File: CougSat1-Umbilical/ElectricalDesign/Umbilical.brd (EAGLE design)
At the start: 49 x 48 mm, 54 parts, among them J1 USB, J2 Umbilical, J3 5V input, Q1 CSD16406Q3, Q2 CSD16406Q3, U1 FT230XQ, U2 BQ24650

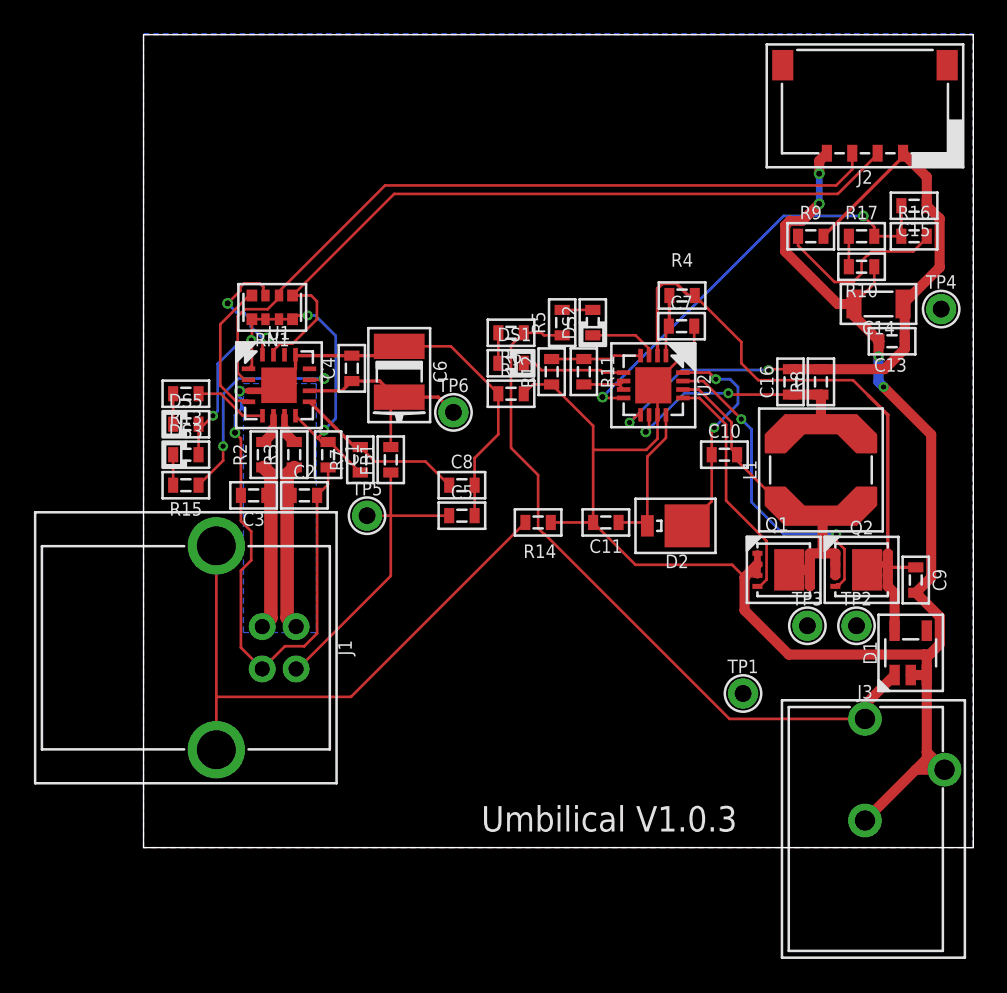
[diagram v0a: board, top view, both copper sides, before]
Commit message: Updated Umbilical
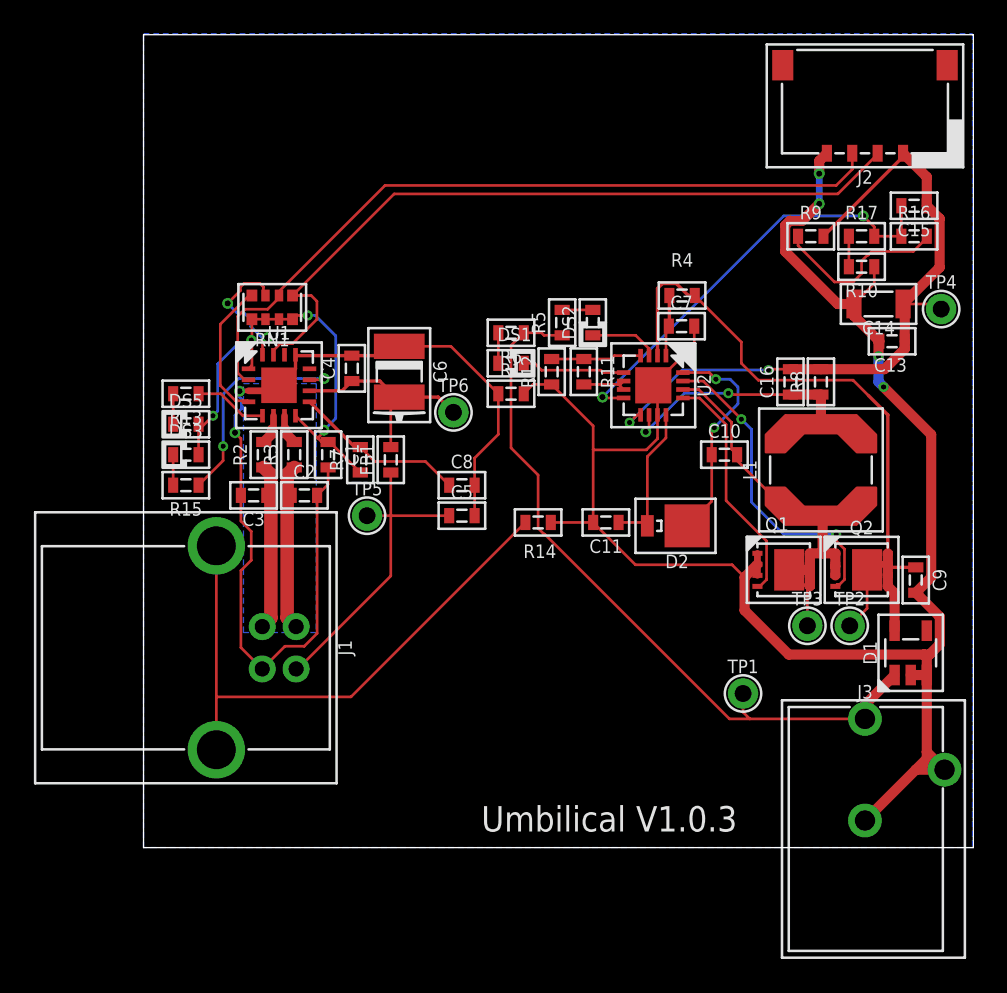
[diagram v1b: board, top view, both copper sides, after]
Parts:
- moved TP2 0.40 mm to (41.7, 13.1)
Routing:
- net PH: track 21.6 -> 25.6 mm
- net DIODE_OUT: track 39.2 -> 42.9 mm
- net UMB_OUT: track 39.2 -> 41.6 mm
- net 5.0V: track 42.4 -> 43.8 mm
- removed copper zone on layer 1, net BALANCING-TOP
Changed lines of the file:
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@@
 <attribute name="NAME" x="35.4" y="10.7" size="0.8" layer="25" font="vector" ratio="15" align="center"/>
 </element>
-<element name="TP2" library="CougsInSpace-Connectors" package="THT-1.0" value="TEST_POINT-THT-1.0" x="42.1" y="13.1" smashed="yes">
-<attribute name="NAME" x="42.1" y="14.7" size="0.8" layer="25" font="vector" ratio="15" align="center"/>
+<element name="TP2" library="CougsInSpace-Connectors" package="THT-1.0" value="TEST_POINT-THT-1.0" x="41.7" y="13.1" smashed="yes">
+<attribute name="NAME" x="41.7" y="14.7" size="0.8" layer="25" font="vector" ratio="15" align="center"/>
 </element>
 <element name="TP3" library="CougsInSpace-Connectors" package="THT-1.0" value="TEST_POINT-THT-1.0" x="39.2" y="13.1" smashed="yes">
@@
 <wire x1="35.3" y1="28.6" x2="36.3" y2="27.6" width="0.16" layer="1"/>
 <wire x1="36.3" y1="27.6" x2="41.9" y2="27.6" width="0.16" layer="1"/>
-<wire x1="42.1" y1="13.1" x2="44.35" y2="12.81" width="0" layer="19" extent="1-1"/>
+<wire x1="42.725" y1="16.4" x2="42.725" y2="14.125" width="0.16" layer="1"/>
+<wire x1="42.725" y1="14.125" x2="41.7" y2="13.1" width="0.16" layer="1"/>
 </signal>
 <signal name="BTST">
@@
 <contactref element="J3" pad="1"/>
 <contactref element="TP1" pad="1"/>
-<wire x1="44.35" y1="10.19" x2="44.26" y2="10.1" width="0.4" layer="1"/>
-<wire x1="22.57" y1="30.4" x2="22.45" y2="30.4" width="0.16" layer="1"/>
 <wire x1="42.6" y1="7.6" x2="42.6" y2="8.44" width="0.6" layer="1"/>
 <wire x1="42.6" y1="8.44" x2="44.35" y2="10.19" width="0.6" layer="1"/>
@@
 <wire x1="23.5" y1="30.4" x2="23.65" y2="30.25" width="0.16" layer="1"/>
 <wire x1="22.45" y1="30.4" x2="23.5" y2="30.4" width="0.16" layer="1"/>
-<wire x1="42.6" y1="7.6" x2="34.6" y2="7.6" width="0.16" layer="1"/>
+<wire x1="42.6" y1="7.6" x2="35.8" y2="7.6" width="0.16" layer="1"/>
+<wire x1="35.8" y1="7.6" x2="34.6" y2="7.6" width="0.16" layer="1"/>
 <wire x1="23.69" y1="18.51" x2="23.6505875" y2="18.51" width="0.16" layer="1"/>
 <wire x1="23.6505875" y1="18.51" x2="23.3" y2="18.8605875" width="0.16" layer="1"/>
@@
 <wire x1="23.3" y1="22" x2="21.7" y2="23.6" width="0.16" layer="1"/>
 <wire x1="21.7" y1="23.6" x2="21.7" y2="29.65" width="0.16" layer="1"/>
-<wire x1="42.6" y1="7.6" x2="35.4" y2="9.1" width="0" layer="19" extent="1-1"/>
+<wire x1="35.8" y1="7.6" x2="35.4" y2="8" width="0.16" layer="1"/>
+<wire x1="35.4" y1="8" x2="35.4" y2="9.1" width="0.16" layer="1"/>
 </signal>
 <signal name="CHARGING_STAT_G">
@@
 <contactref element="TP3" pad="1"/>
 <wire x1="40" y1="19.6" x2="39.0401875" y2="19.6" width="0.4" layer="1"/>
-<wire x1="40.85" y1="17.375" x2="40.85" y2="16.075" width="0.6" layer="1"/>
-<wire x1="39.35" y1="17.375" x2="39.35" y2="16.4" width="0.6" layer="1"/>
-<wire x1="39.35" y1="16.4" x2="39.35" y2="15.425" width="0.6" layer="1"/>
+<wire x1="40.85" y1="17.375" x2="40.85" y2="16.6" width="0.6" layer="1"/>
+<wire x1="40.85" y1="16.6" x2="40.85" y2="16.075" width="0.6" layer="1"/>
+<wire x1="39.35" y1="17.375" x2="39.35" y2="16.8" width="0.6" layer="1"/>
+<wire x1="39.35" y1="16.8" x2="39.35" y2="16.4" width="0.6" layer="1"/>
+<wire x1="39.35" y1="15.425" x2="39.35" y2="16" width="0.6" layer="1"/>
+<wire x1="39.35" y1="16" x2="39.35" y2="16.4" width="0.6" layer="1"/>
 <wire x1="38.125" y1="16.4" x2="39.35" y2="16.4" width="0.6" layer="1"/>
 <wire x1="40.85" y1="17.375" x2="40.1" y2="17.375" width="0.6" layer="1"/>
@@
 <wire x1="34.72" y1="23.53" x2="34.72" y2="25.11631875" width="0.16" layer="1"/>
 <wire x1="34.72" y1="25.11631875" x2="32.78631875" y2="27.05" width="0.16" layer="1"/>
-<wire x1="40.85" y1="16.075" x2="40.85" y2="16.725" width="0" layer="19" extent="1-1"/>
-<wire x1="39.35" y1="16.075" x2="39.35" y2="15.425" width="0" layer="19" extent="1-1"/>
-<wire x1="39.35" y1="16.725" x2="39.35" y2="17.375" width="0" layer="19" extent="1-1"/>
-<wire x1="39.2" y1="13.1" x2="39.35" y2="15.425" width="0" layer="19" extent="1-1"/>
+<wire x1="38.125" y1="16.4" x2="39.2" y2="15.325" width="0.16" layer="1"/>
+<wire x1="39.2" y1="15.325" x2="39.2" y2="13.1" width="0.16" layer="1"/>
+<wire x1="40.85" y1="16.725" x2="40.85" y2="16.6" width="0.16" layer="1"/>
+<wire x1="39.35" y1="16.725" x2="39.35" y2="16.8" width="0.16" layer="1"/>
+<wire x1="39.35" y1="16.075" x2="39.35" y2="16" width="0.16" layer="1"/>
 </signal>
 <signal name="HIGHDV">
@@
 <wire x1="36.9" y1="28.2" x2="36.95" y2="28.25" width="0.16" layer="1"/>
 <wire x1="36.95" y1="28.25" x2="38.2" y2="28.25" width="0.16" layer="1"/>
-<wire x1="44.85" y1="32.1" x2="47.1" y2="31.8" width="0" layer="19" extent="1-1"/>
+<wire x1="44.85" y1="32.1" x2="46.8" y2="32.1" width="0.16" layer="1"/>
+<wire x1="46.8" y1="32.1" x2="47.1" y2="31.8" width="0.16" layer="1"/>
 </signal>
 <signal name="UMB_RX">
@@
 <wire x1="10.2875" y1="24.1875" x2="10.525" y2="23.95" width="0.16" layer="1"/>
 <wire x1="10.525" y1="23.95" x2="10.9" y2="23.95" width="0.16" layer="1"/>
-<wire x1="6.4" y1="31.2" x2="6.4" y2="28.475" width="0.16" layer="1"/>
+<wire x1="6.4" y1="28.475" x2="6.4" y2="30.2" width="0.16" layer="1"/>
+<wire x1="6.4" y1="30.2" x2="6.4" y2="31.2" width="0.16" layer="1"/>
 <wire x1="6.4" y1="28.475" x2="6.2" y2="28.275" width="0.16" layer="1"/>
 <wire x1="12.8" y1="22.15" x2="11" y2="23.95" width="0.16" layer="1"/>
@@
 <wire x1="9.025" y1="31.425" x2="8.8" y2="31.2" width="0.16" layer="1"/>
 <wire x1="11.35" y1="30.2187375" x2="10.1437375" y2="31.425" width="0.16" layer="16"/>
-<wire x1="6.4" y1="30.1" x2="6.4" y2="31.2" width="0" layer="19" extent="1-1"/>
+<wire x1="6.365" y1="29.97131875" x2="6.365" y2="30.165" width="0.16" layer="1"/>
+<wire x1="6.365" y1="30.165" x2="6.4" y2="30.2" width="0.16" layer="1"/>
 </signal>
 <signal name="DGND">
@@
 </signal>
 <signal name="BALANCING-TOP">
-<polygon width="0.16" layer="1" spacing="0.5" pour="hatch" rank="6">
-<vertex x="0" y="0"/>
-<vertex x="0" y="48"/>
-<vertex x="49" y="48"/>
-<vertex x="49" y="0"/>
-</polygon>
 </signal>
 <signal name="CBUS1">
